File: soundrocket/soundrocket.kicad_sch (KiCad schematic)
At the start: 11 parts, among them J1 XLR3 MALE (OUT), SW1 SW_Push, SW2 RotaryEncoder_Switch, T1 PE-65612NL, U1 Teensy4.0, U2 DIT4192IPW, U3 TPS63061

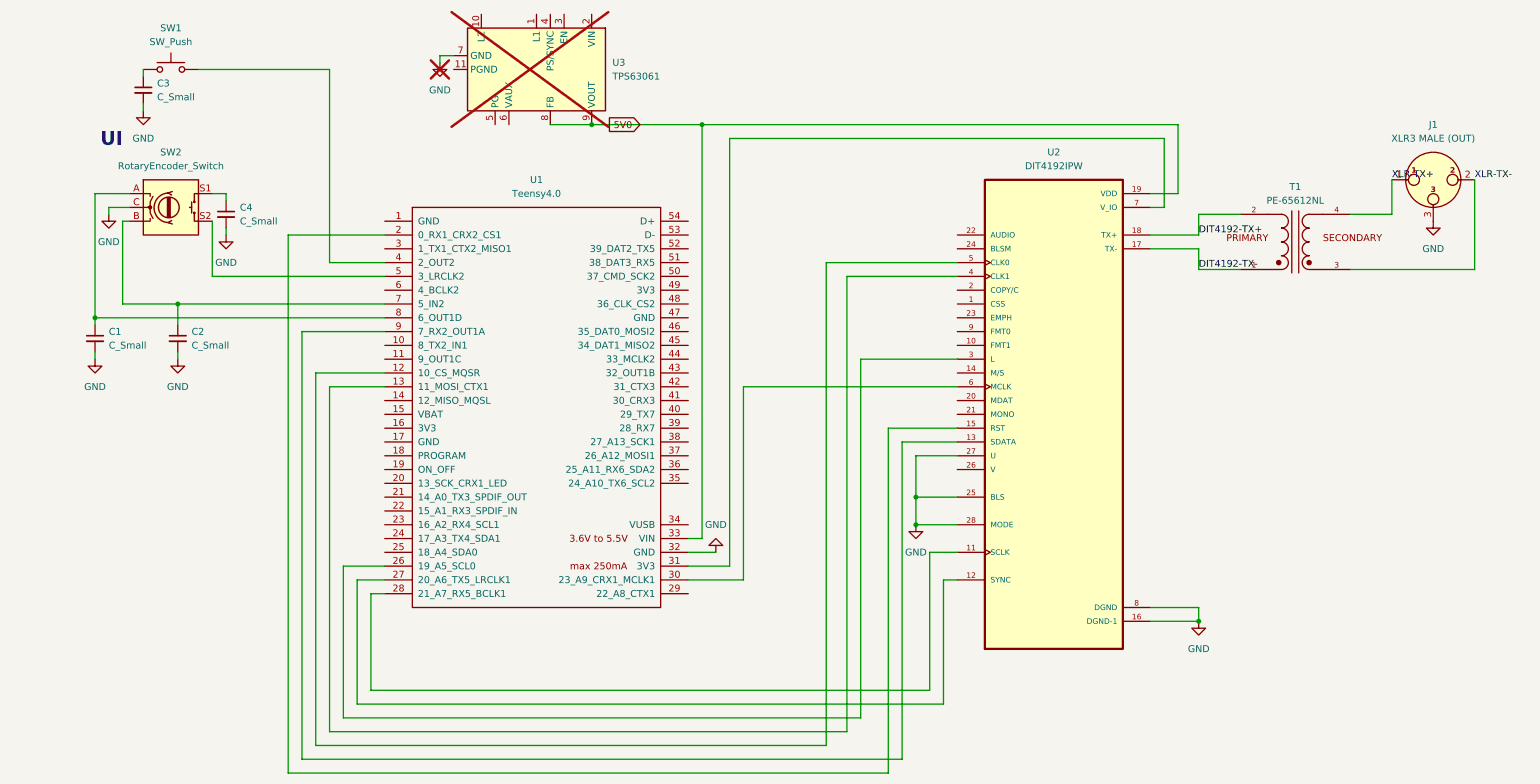
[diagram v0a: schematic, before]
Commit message: Hardware Test & Revision 2
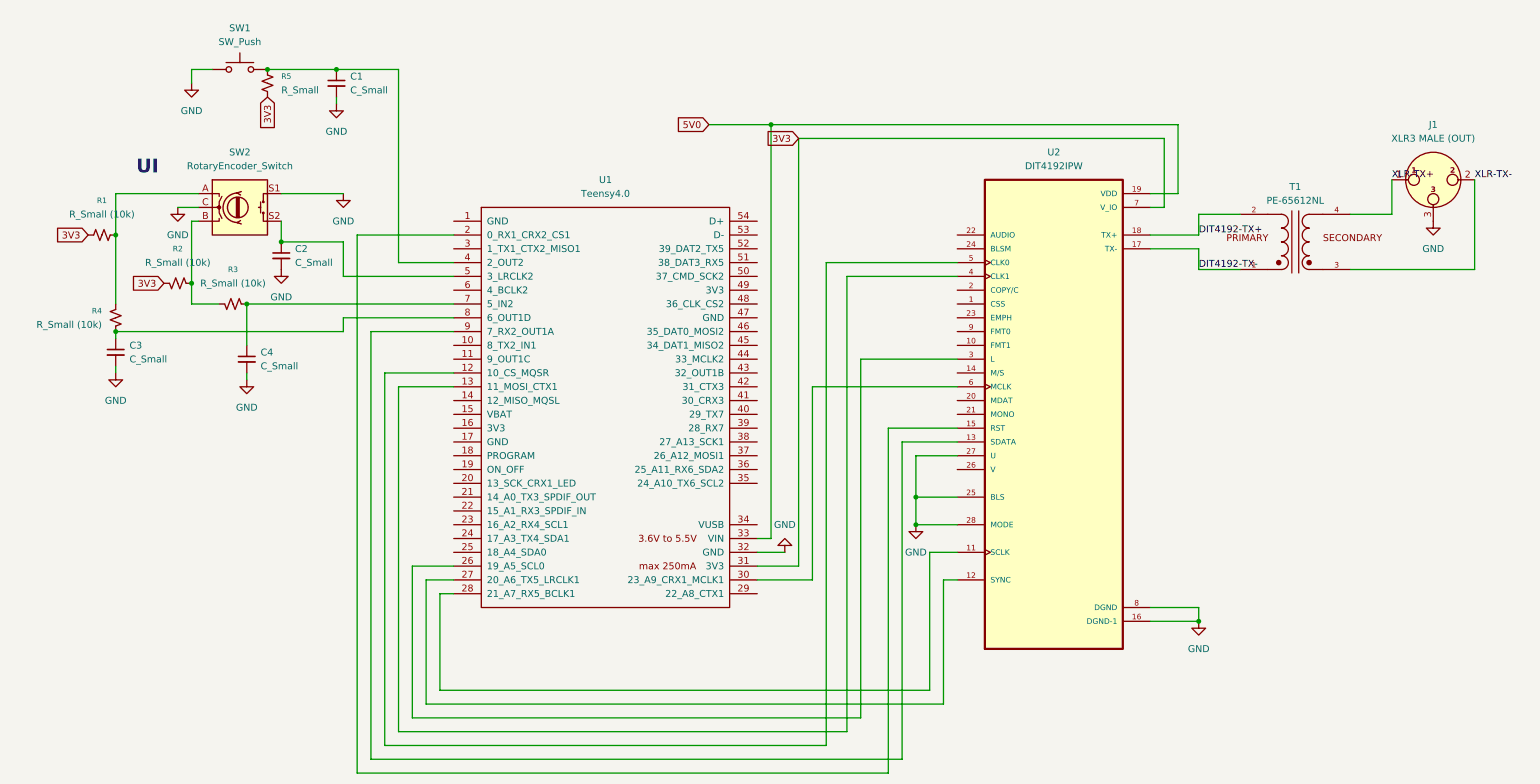
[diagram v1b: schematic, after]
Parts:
- removed U3: TPS63061, Package_SON:Texas_S-PWSON-N10_ThermalVias, symbol Regulator_Switching:TPS63061
- added R1, R2, R3, R4: R_Small (10k), KiCad Models:STA_CF14_STP, symbol Device:R_Small_US
- added R5: R_Small, KiCad Models:STA_CF14_STP, symbol Device:R_Small_US
- J1: footprint Connector_Audio:Jack_XLR_Neutrik_NC3FAAH-0_Horizontal -> Connector_Audio:Jack_XLR_Neutrik_NC3MAAV_Vertical
- renumbered C3 to C1, C4 to C2, C1 to C3, C2 to C4
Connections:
- net GND: now also SW1.1, SW2.S1
- net at C1.1: now also SW1.2, U1.4 (2_OUT2), R5.1; no longer SW1.1
- net at C2.1: now also SW2.S2, U1.5 (3_LRCLK2); no longer SW2.S1
- net at C4.1, U1.7 (5_IN2): now also R3.1; no longer SW2.B
- net at C3.1, U1.8 (6_OUT1D): now also R4.1; no longer SW2.A
- net 3V3: now reaches U1.31 (3V3), U2.7 (V_IO)
- net 3V3: now also R1.2, R2.2, R5.2
- new net: R2.1, R3.2, SW2.B
- new net: R1.1, R4.2, SW2.A
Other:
- moved on the sheet: C1, C2, C3, C4, SW1, SW2, U1
